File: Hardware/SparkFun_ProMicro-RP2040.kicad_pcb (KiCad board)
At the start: 4 copper layers, 25 x 25 mm, 44 parts, among them J1 Conn_01x12_Male, J2 Qwiic, J3 Conn_01x12_Male, J4 Conn_01x04_Male, U1 3.3V, U2 RP2040, U3 WS2812-2020, U4 W25QXX128MBIT, Y1 12MHz

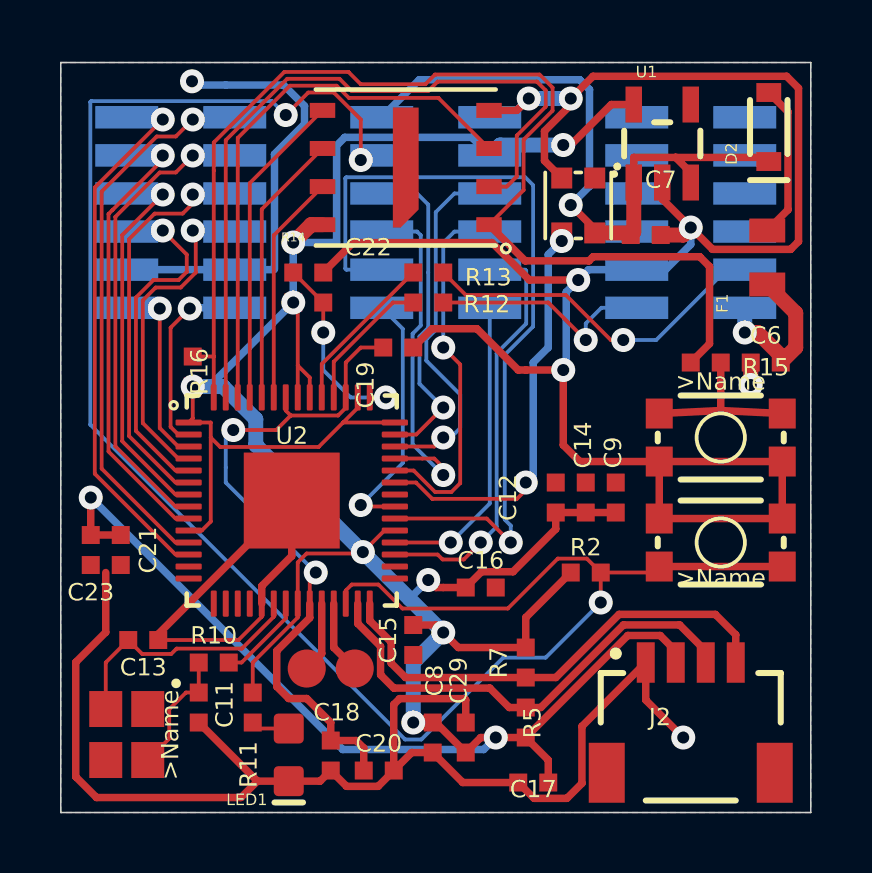
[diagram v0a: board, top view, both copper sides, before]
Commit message: .
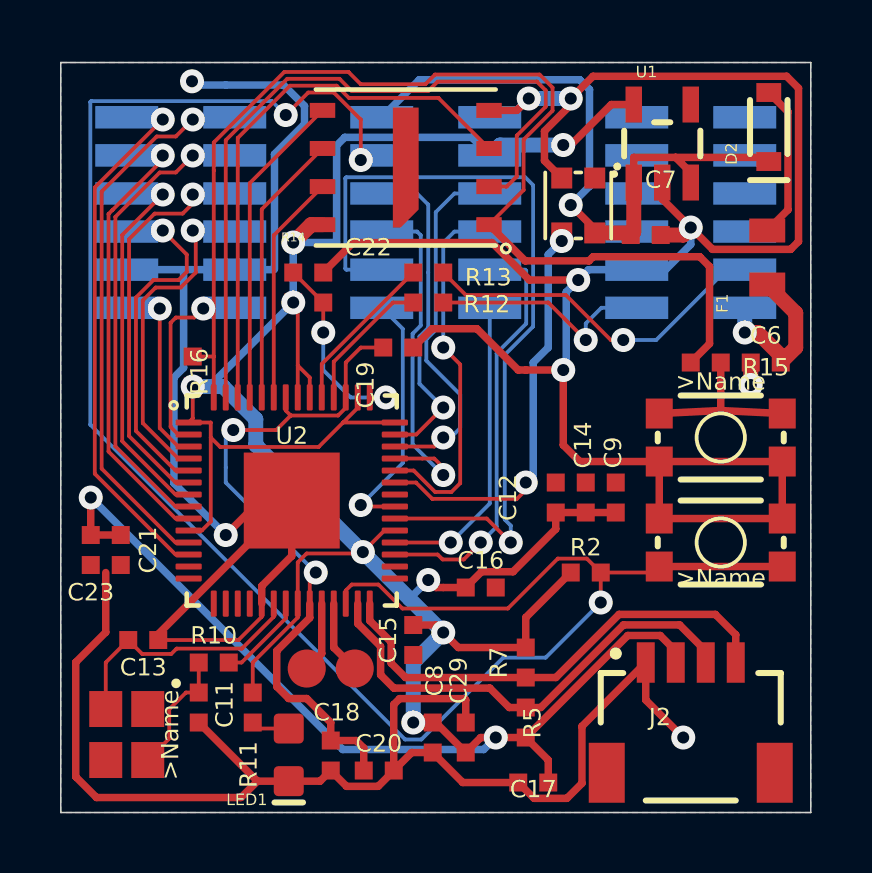
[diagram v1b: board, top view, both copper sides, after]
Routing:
- net GND: track 141.9 -> 154.3 mm, vias 8 -> 9
- net /0/TX0: track 6.43 -> 5.46 mm
